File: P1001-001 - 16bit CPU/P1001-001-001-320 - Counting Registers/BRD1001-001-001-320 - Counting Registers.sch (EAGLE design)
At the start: 15 parts, among them IC1 74HC192D, IC12 74AC245DW, IC2 74HC192D, IC27 MEGA8535-A, IC3 74HC192D, IC4 74HC192D, IC7 74AC245DW, J1 22-27-2041-04

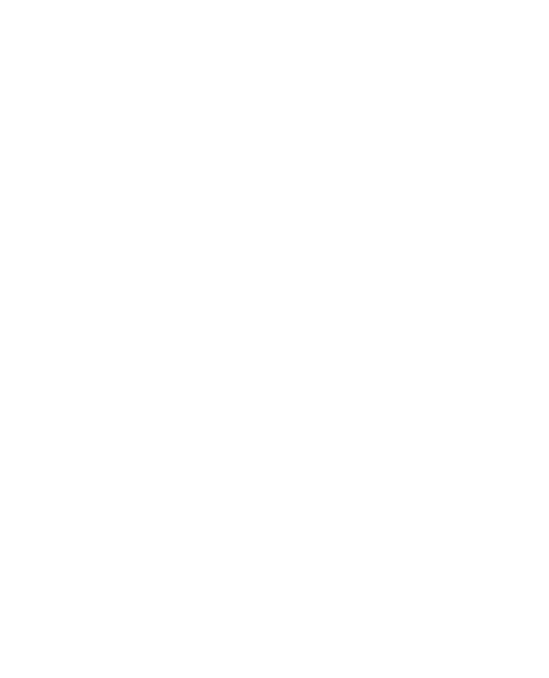
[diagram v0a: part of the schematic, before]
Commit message: Finished All Boards
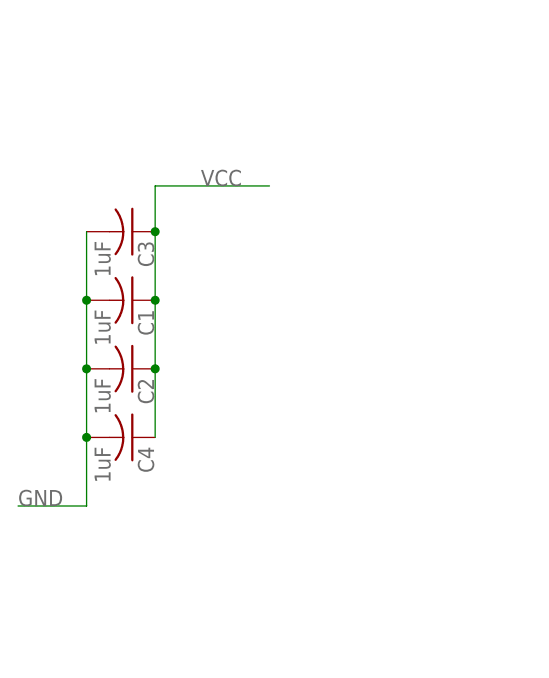
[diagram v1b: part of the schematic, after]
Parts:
- added C1, C2, C3, C4: 1uF, rcl:C-USC1206
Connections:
- net GND: now also C1.2, C2.2, C3.2, C4.2
- net VCC: now also C1.1, C2.1, C3.1, C4.1
